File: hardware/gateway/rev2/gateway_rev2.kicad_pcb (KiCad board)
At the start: 2 copper layers, 100 x 45 mm, 80 parts, among them IC1 STM8L151K4T6, IC2 CC1101RGPR, IC3 LT1615ES5-1#TRMPBF, IC4 MIC4427YM, IC5 MB85RC64TAPNF-G-BDERE1, J1 G8250041000YEU, J2 M20-9770342, Q1 IRLML6402TRPBF, U1 2462, Y1 NX3225GA-26.000M-STD-CRG-2

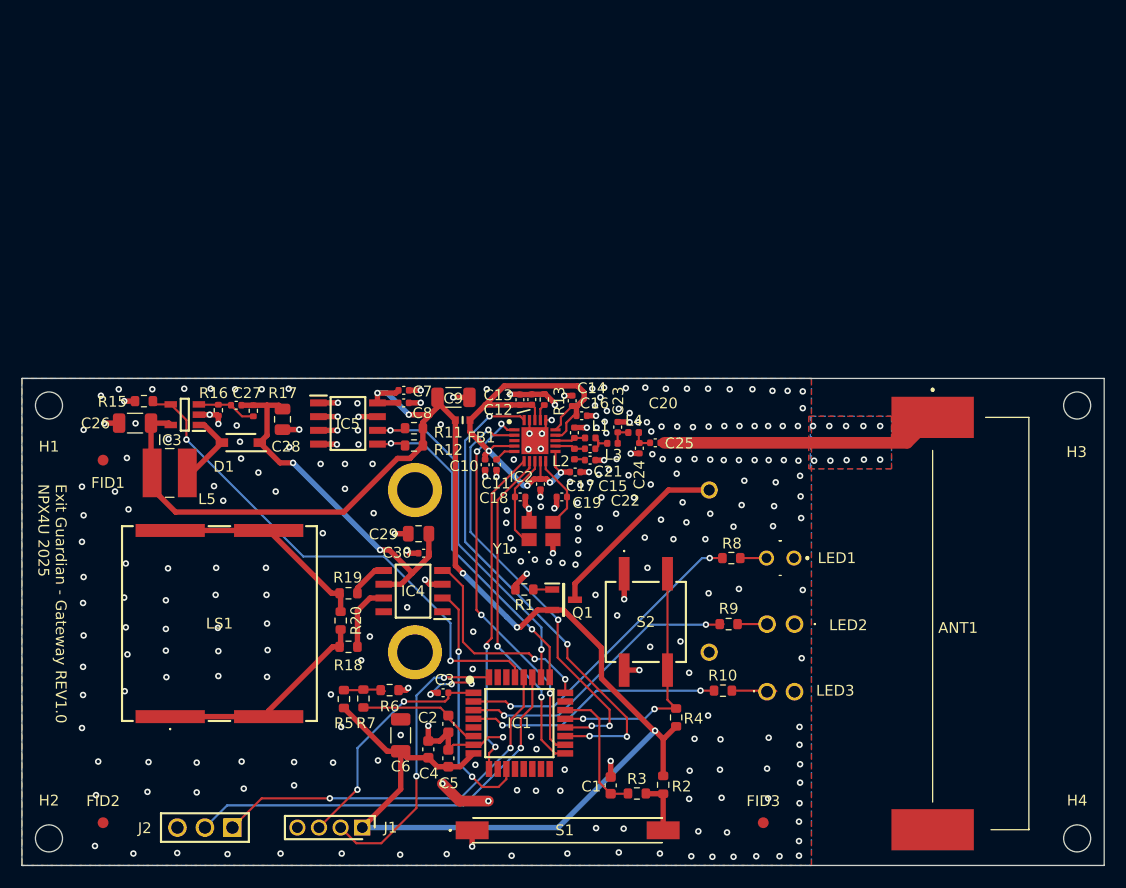
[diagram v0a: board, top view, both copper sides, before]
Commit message: EG-59 Schematic with the needed components, plus PCB.
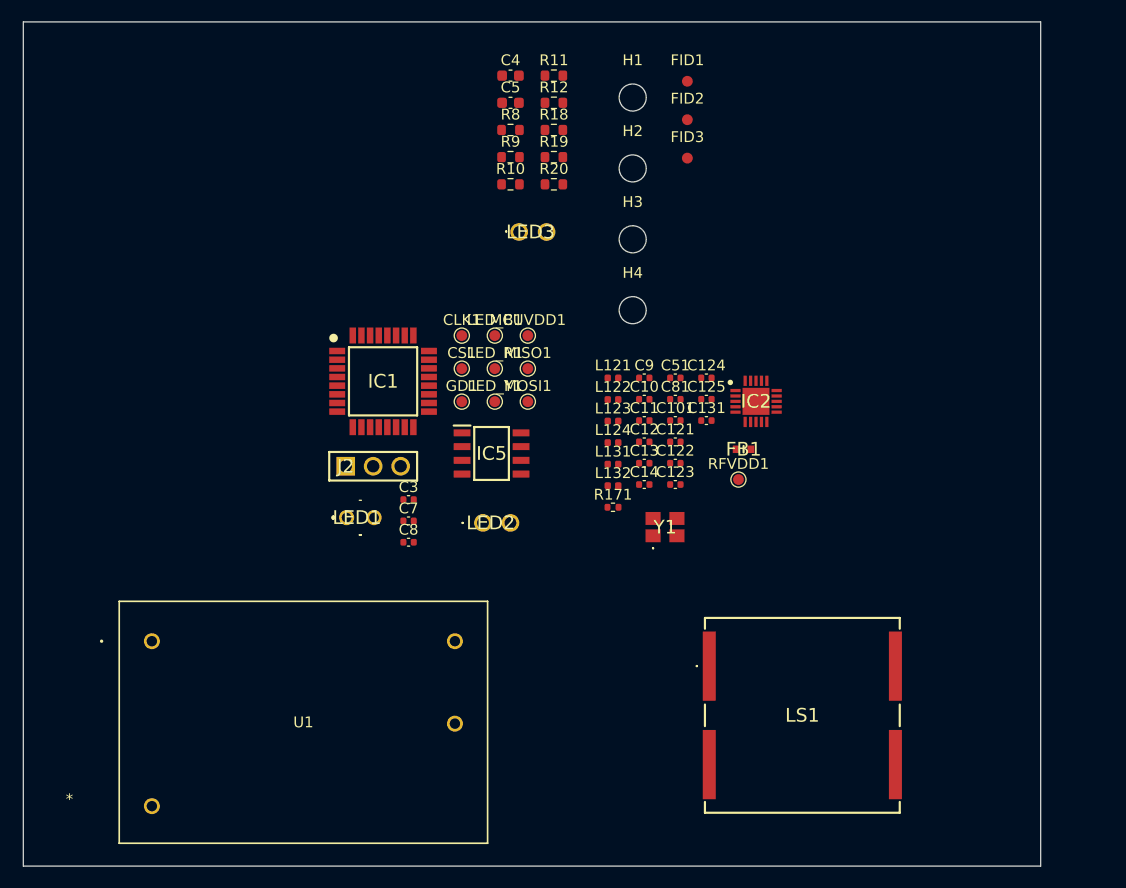
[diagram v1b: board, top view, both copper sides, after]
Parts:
- removed ANT1: ANT-433-HESM, MyParts:ANT433HESM
- removed C1, C2: 100nF, Capacitor_SMD:C_0603_1608Metric
- removed C15, C16, C17, C30: 100nF, Capacitor_SMD:C_0402_1005Metric
- removed C18, C19: 12pF, Capacitor_SMD:C_0402_1005Metric
- removed C20, C22: 3.9pF, Capacitor_SMD:C_0402_1005Metric
- removed C21, C25: 220pF, Capacitor_SMD:C_0402_1005Metric
- removed C23: 8.2pF, Capacitor_SMD:C_0402_1005Metric
- removed C24: 5.6pF, Capacitor_SMD:C_0402_1005Metric
- removed C26: 22uF, 6.3V, Capacitor_SMD:C_1206_3216Metric
- removed C27: 4.7pF, Capacitor_SMD:C_0402_1005Metric
- removed C28, C29: 4.7uF, 25V, Capacitor_SMD:C_0805_2012Metric
- removed C6: 47uF, 6.3V, Capacitor_SMD:C_1206_3216Metric
- removed D1: MBR0520LT3G, MyParts:SOD3716X135N
- removed IC3: LT1615ES5-1#TRMPBF, MyParts:SOT95P280X100-5N
- removed IC4: MIC4427YM, MyParts:SOIC127P599X173-8N
- removed J1: G8250041000YEU, MyParts:HDRV4W55P0X200_1X4_800X200X635P
- removed L1, L2, L4: 27nH, Inductor_SMD:L_0402_1005Metric
- removed L3: 22nH, Inductor_SMD:L_0402_1005Metric
- removed L5: CD43NP-100MC, MyParts:CD43NP100MC
- removed Q1: IRLML6402TRPBF, MyParts:SOT95P237X112-3N
- removed R1, R15, R3: 100K, Resistor_SMD:R_0603_1608Metric
- removed R13: 56K, Resistor_SMD:R_0402_1005Metric
- removed R16: 130K, Resistor_SMD:R_0402_1005Metric
- removed R17: 1.15M, Resistor_SMD:R_0402_1005Metric
- removed R2, R5: 1M, Resistor_SMD:R_0603_1608Metric
- removed R4: 10K, Resistor_SMD:R_0603_1608Metric
- removed R6: 510K, Resistor_SMD:R_0603_1608Metric
- removed R7: 1K, Resistor_SMD:R_0603_1608Metric
- removed S1: MASM-14R-8-10, MyParts:MASM14R810
- removed S2: TL6120DF160QG, MyParts:TL6120DF160QG
- added C101: 15pF, Capacitor_SMD:C_0402_1005Metric, F.Cu at (239.9, 118.8)
- added C121: 1pF, Capacitor_SMD:C_0402_1005Metric, F.Cu at (239.9, 120.8)
- added C122: 1.5pF, Capacitor_SMD:C_0402_1005Metric, F.Cu at (239.9, 122.8)
- added C123: 3.3pF, Capacitor_SMD:C_0402_1005Metric, F.Cu at (239.9, 124.8)
- added C124: 100pF, Capacitor_SMD:C_0402_1005Metric, F.Cu at (242.7, 114.9)
- added C125: 12pF, Capacitor_SMD:C_0402_1005Metric, F.Cu at (242.7, 116.9)
- added C131: 1.5pF, Capacitor_SMD:C_0402_1005Metric, F.Cu at (242.7, 118.8)
- added C51: 100nF, Capacitor_SMD:C_0402_1005Metric, F.Cu at (239.9, 114.9)
- added C81: 15pF, Capacitor_SMD:C_0402_1005Metric, F.Cu at (239.9, 116.9)
- added CLK1: SPI_CK, TestPoint:TestPoint_Pad_D1.0mm, F.Cu at (220.1, 111.0)
- added CS1: SPI_CS, TestPoint:TestPoint_Pad_D1.0mm, F.Cu at (220.1, 114.0)
- added GD1: GD0, TestPoint:TestPoint_Pad_D1.0mm, F.Cu at (220.1, 117.1)
- added L121: 12nH, Inductor_SMD:L_0402_1005Metric, F.Cu at (234.1, 114.9)
- added L122: 18nH, Inductor_SMD:L_0402_1005Metric, F.Cu at (234.1, 116.9)
- added L123: 12nH, Inductor_SMD:L_0402_1005Metric, F.Cu at (234.1, 118.9)
- added L124: 12nH, Inductor_SMD:L_0402_1005Metric, F.Cu at (234.1, 120.9)
- added L131: 12nH, Inductor_SMD:L_0402_1005Metric, F.Cu at (234.1, 122.9)
- added L132: 18nH, Inductor_SMD:L_0402_1005Metric, F.Cu at (234.1, 124.9)
- added LED_B1: LED, TestPoint:TestPoint_Pad_D1.0mm, F.Cu at (223.2, 111.0)
- added LED_R1: LED, TestPoint:TestPoint_Pad_D1.0mm, F.Cu at (223.2, 114.0)
- added LED_Y1: LED, TestPoint:TestPoint_Pad_D1.0mm, F.Cu at (223.2, 117.1)
- added MCUVDD1: MCU_VDD, TestPoint:TestPoint_Pad_D1.0mm, F.Cu at (226.2, 111.0)
- added MISO1: SPI_MISO, TestPoint:TestPoint_Pad_D1.0mm, F.Cu at (226.2, 114.0)
- added MOSI1: SPI_MOSI, TestPoint:TestPoint_Pad_D1.0mm, F.Cu at (226.2, 117.1)
- added R171: 56K, Resistor_SMD:R_0402_1005Metric, F.Cu at (234.1, 126.9)
- added RFVDD1: RF_VDD, TestPoint:TestPoint_Pad_D1.0mm, F.Cu at (245.7, 124.3)
- C13: value 1uF -> 100nF
- C9: value 47uF, 6.3V -> 100nF; footprint Capacitor_SMD:C_1206_3216Metric -> Capacitor_SMD:C_0402_1005Metric
- R18, R19: value 33R -> 100R
- R20: value 1M -> 10K
- U1: value 2462 -> IRM-01-3.3; footprint MyParts:2462 -> MyParts:IRM-01-3-3; moved to F.Cu
- Y1: value NX3225GA-26.000M-STD-CRG-2 -> NX3225GA-26MHZ-TI
- moved FID2 84.5 mm to (241.0, 91.0)
- moved H2 82.1 mm to (235.9, 95.5)
- moved FID1 64.3 mm to (241.0, 87.5)
- moved H4 63.8 mm to (235.9, 108.6)
- moved C4 62.7 mm to (224.6, 87.0), turned to 0 degrees
- moved FID3 61.8 mm to (241.0, 94.6)
- moved H1 61.0 mm to (235.9, 89.0)
- moved C5 60.8 mm to (224.6, 89.5), turned to 0 degrees
- moved U1 59.2 mm to (191.5, 154.5)
- moved LS1 54.5 mm to (251.6, 146.1), turned to 0 degrees
- moved R18 51.4 mm to (228.7, 92.0)
- moved R10 50.7 mm to (224.6, 97.0)
- moved LED3 48.3 mm to (225.4, 101.4)
- moved R9 47.6 mm to (224.6, 94.5)
- moved R20 44.9 mm to (228.7, 97.0), turned to 0 degrees
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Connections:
- C11 pad 1: Net-(IC2-DCOUPL) -> RF_VDD
- C9 pad 1: VDD -> RF_VDD
- FB1 pad 1: VDD -> RF_VDD
- FB1 pad 2: RF_VDD -> VDD
- IC1 pad 11: /Buzzer/BZR_P -> BZR_P
- IC1 pad 22: DOOR -> unconnected-(IC1-PD5-Pad22)
- IC1 pad 24: /Buzzer/BZR_N -> BZR_N
- IC1 pad 29: /Buzzer/BZR_EN -> unconnected-(IC1-PC4-Pad29)
- IC1 pad 6: V_MEAS -> unconnected-(IC1-PA6-Pad6)
- J2 pad 1: TX -> GND
- J2 pad 3: GND -> TX
- R18 pad 2: Net-(IC4-OUTA) -> BZR_P
- R19 pad 2: Net-(IC4-OUTB) -> BZR_N
- U1 pad 1: BAT_IN -> unconnected-(U1-AC/L-Pad1)
- Y1 pad 2: GND -> unconnected-(Y1-NC/GND_1-Pad2)
- Y1 pad 4: GND -> unconnected-(Y1-NC/GND_2-Pad4)
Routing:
- net VDD: track 157.1 -> 0.00 mm, vias 5 -> 0
- net GND: track 80.1 -> 0.00 mm, vias 287 -> 0
- net /Buzzer/BZR_EN: track 47.7 -> 0.00 mm, vias 2 -> 0
- net RF_VDD: track 47.6 -> 0.00 mm, vias 4 -> 0
- net /MCU/SDI: track 45.8 -> 0.00 mm, vias 4 -> 0
- net /MCU/SDO: track 40.2 -> 0.00 mm, vias 4 -> 0
- net RX: track 39.2 -> 0.00 mm, vias 1 -> 0
- net /MCU/SCLK: track 36.0 -> 0.00 mm, vias 4 -> 0
- net TX: track 35.8 -> 0.00 mm, vias 2 -> 0
- net +12V: track 34.3 -> 0.00 mm, vias 2 -> 0
- net SCL: track 33.5 -> 0.00 mm, vias 2 -> 0
- net SDA: track 32.1 -> 0.00 mm, vias 2 -> 0
- net /MCU/CS: track 31.4 -> 0.00 mm, vias 2 -> 0
- net /MCU/IRQ: track 30.5 -> 0.00 mm, vias 2 -> 0
- net LED_B: track 28.9 -> 0.00 mm, vias 2 -> 0
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- removed copper zone on B.Cu, net GND
- removed copper zone on F.Cu, net GND
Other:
- board size 100 x 45 mm -> 94 x 78 mm
- board text removed: "Exit Guardian - Gateway REV1.0 NPX4U 2025"
